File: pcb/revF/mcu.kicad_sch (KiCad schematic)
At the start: 64 parts, among them CON1 JOYSTICK, CON2 KEYBOARD, CON3 MOUSE, Q1 IRLML2402, Q2 IRLML2402, Q3 IRLML2402, Q4 IRLML2402, U4 24LC08B, U5 W25Q128JVS, U6 DS3231MZ, U7 LM1117MP-3.3, U8 74HC597, U9 RP2040, Y1 12MHz

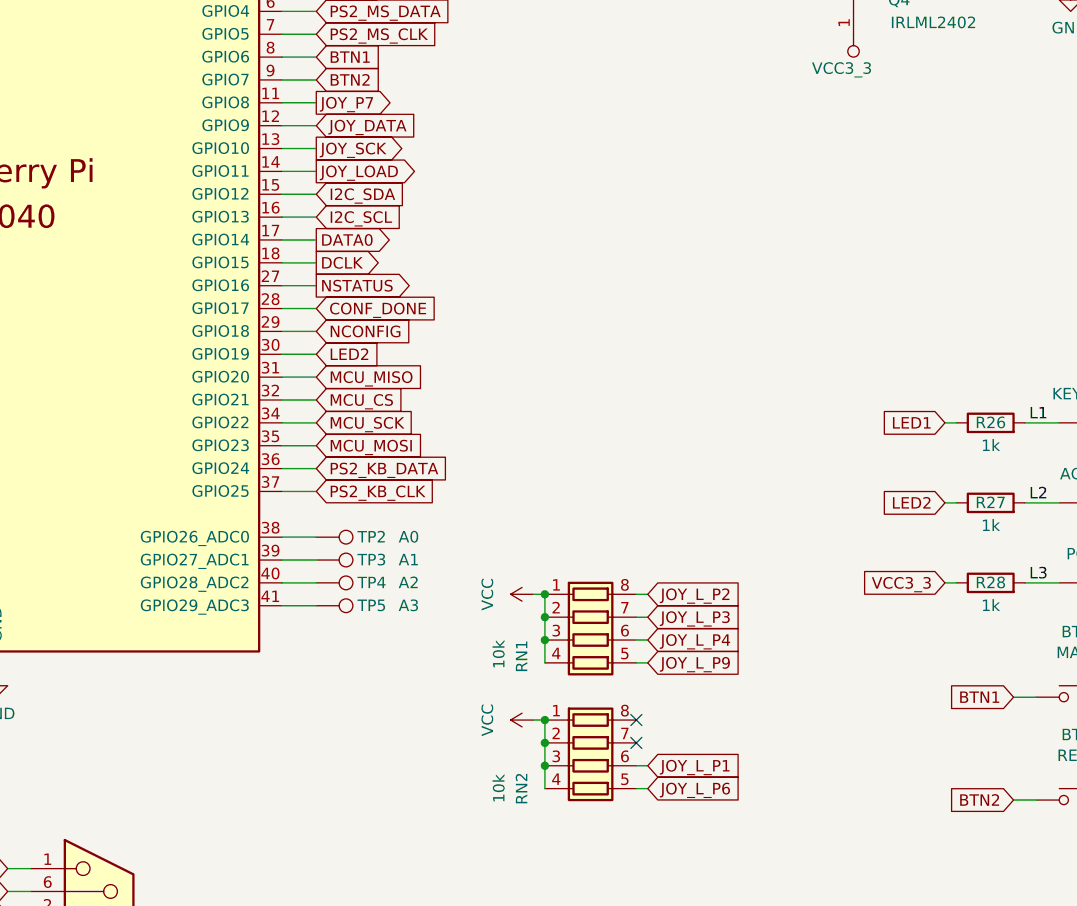
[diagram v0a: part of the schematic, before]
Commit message: RevF pcb
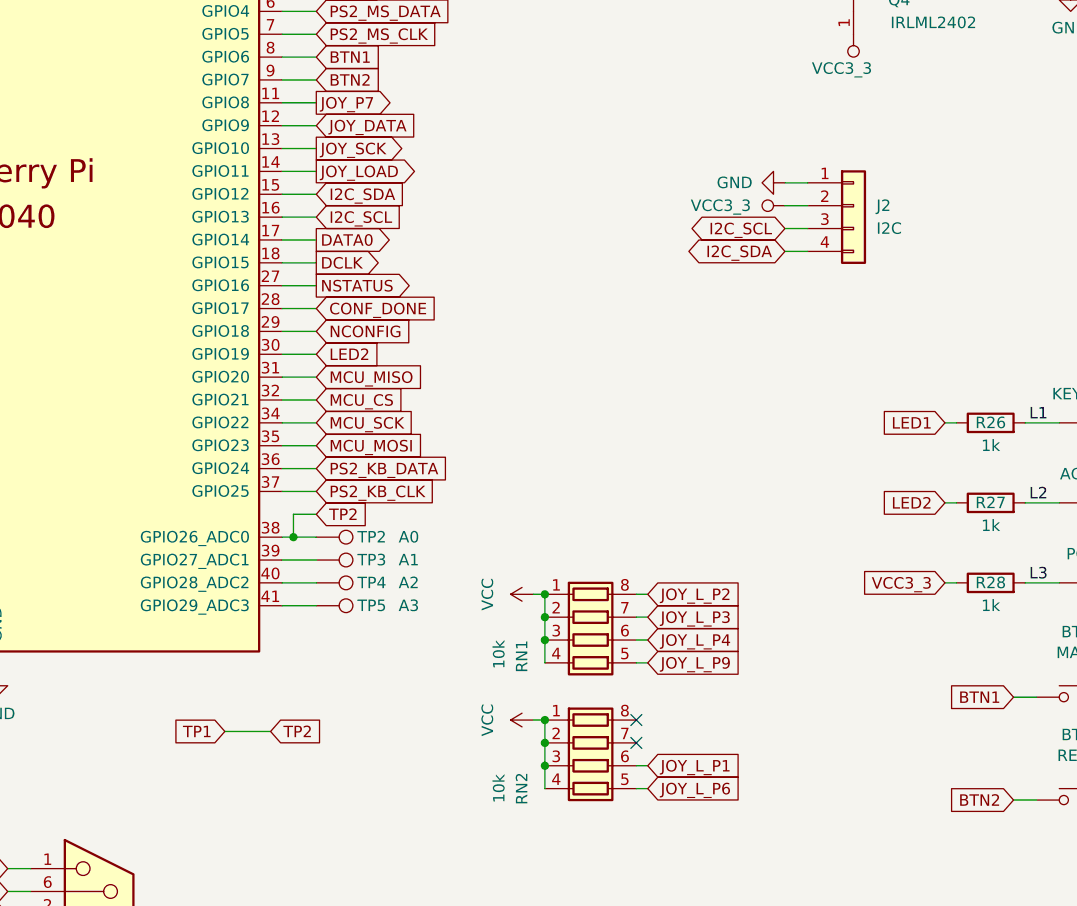
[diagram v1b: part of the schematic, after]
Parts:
- added J2: I2C, Connector_PinHeader_2.54mm:PinHeader_1x04_P2.54mm_Vertical, symbol Connector_Generic:Conn_01x04
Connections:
- net GND: now also J2.1 (Pin_1)
- net I2C_SCL: now also J2.3 (Pin_3)
- net I2C_SDA: now also J2.4 (Pin_4)
- net VCC3_3: now also J2.2 (Pin_2)
- net TP1: now reaches TP2.1, U9.38 (GPIO26_ADC0)

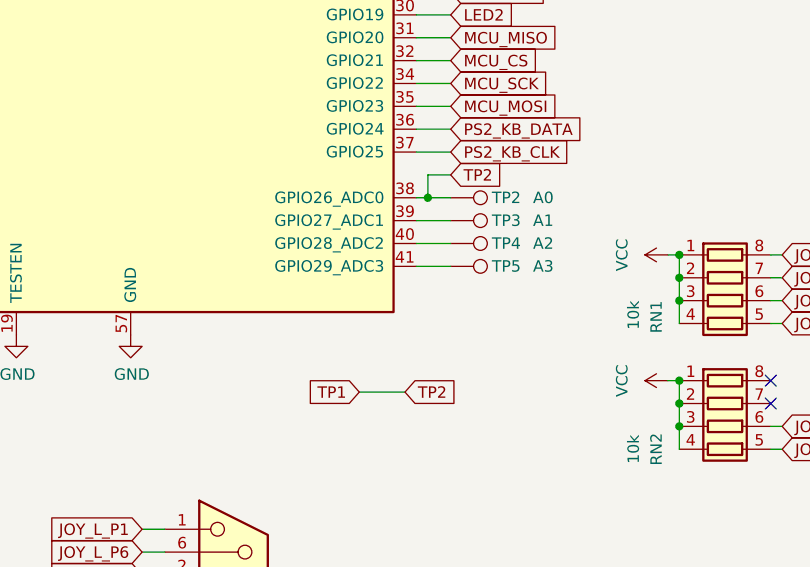
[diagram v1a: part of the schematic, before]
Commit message: Refactored revF alpha2
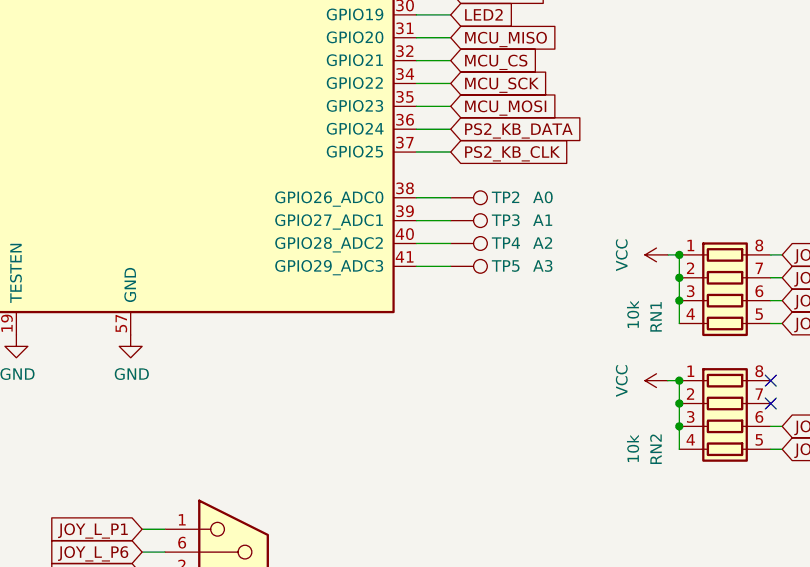
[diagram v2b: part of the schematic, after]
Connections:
- net TP1: no longer names the net of TP2.1, U9.38 (GPIO26_ADC0)
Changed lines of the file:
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@@
 	)
 	(junction
-		(at 181.61 127)
-		(diameter 0)
-		(color 0 0 0 0)
-	)
-	(junction
 		(at 149.86 29.21)
 		(diameter 0)
@@
 	(wire
 		(pts
-			(xy 184.15 124.46) (xy 181.61 124.46)
-		)
-		(stroke
-			(width 0)
-			(type default)
-		)
-	)
-	(wire
-		(pts
 			(xy 154.94 39.37) (xy 154.94 40.64)
 		)
@@
 	(wire
 		(pts
-			(xy 180.34 127) (xy 181.61 127)
+			(xy 180.34 127) (xy 184.15 127)
 		)
 		(stroke
@@
 	(wire
 		(pts
-			(xy 173.99 148.59) (xy 179.07 148.59)
-		)
-		(stroke
-			(width 0)
-			(type default)
-		)
-	)
-	(wire
-		(pts
 			(xy 262.89 114.3) (xy 266.7 114.3)
 		)
@@
 	(wire
 		(pts
-			(xy 181.61 127) (xy 184.15 127)
-		)
-		(stroke
-			(width 0)
-			(type default)
-		)
-	)
-	(wire
-		(pts
 			(xy 114.3 93.98) (xy 116.84 93.98)
 		)
@@
 	(wire
 		(pts
-			(xy 181.61 124.46) (xy 181.61 127)
-		)
-		(stroke
-			(width 0)
-			(type default)
-		)
-	)
-	(wire
-		(pts
 			(xy 180.34 121.92) (xy 184.15 121.92)
 		)
@@
 		)
 	)
-	(global_label "TP1"
-		(shape input)
-		(at 173.99 148.59 180)
-		(fields_autoplaced yes)
-		(effects
-			(font
-				(size 1.27 1.27)
-			)
-			(justify right)
-		)
-		(property "Intersheetrefs" "${INTERSHEET_REFS}"
-			(at 168.2119 148.59 0)
-			(effects
-				(font
-					(size 1.27 1.27)
-				)
-				(justify right)
-				(hide yes)
-			)
-		)
-	)
 	(global_label "JOY_L_P6"
 		(shape input)
@@
 		)
 	)
-	(global_label "TP2"
-		(shape input)
-		(at 179.07 148.59 0)
-		(fields_autoplaced yes)
-		(effects
-			(font
-				(size 1.27 1.27)
-			)
-			(justify left)
-		)
-		(property "Intersheetrefs" "${INTERSHEET_REFS}"
-			(at 184.8481 148.59 0)
-			(effects
-				(font
-					(size 1.27 1.27)
-				)
-				(justify left)
-				(hide yes)
-			)
-		)
-	)
 	(global_label "JOY_P7"
 		(shape output)
@@
 			(effects
 				(font
-					(size 1.27 1.27)
-				)
-				(justify left)
-				(hide yes)
-			)
-		)
-	)
-	(global_label "TP2"
-		(shape input)
-		(at 184.15 124.46 0)
-		(fields_autoplaced yes)
-		(effects
-			(font
-				(size 1.27 1.27)
-			)
-			(justify left)
-		)
-		(property "Intersheetrefs" "${INTERSHEET_REFS}"
-			(at 189.9281 124.46 0)
-			(effects
-				(font
